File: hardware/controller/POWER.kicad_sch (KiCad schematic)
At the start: 22 parts, among them IC101 TPS63000IDRCRQ1, J101 1769

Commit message: done but need to add stitching vias
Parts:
- TP101, TP102, TP103, TP104, TP105: footprint TestPoint:TestPoint_Pad_1.0x1.0mm -> SamacSys_Parts:TestPoint_Pad_1.0x1.0mm
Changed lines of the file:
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@@
 			)
 		)
-		(property "Footprint" "TestPoint:TestPoint_Pad_1.0x1.0mm"
+		(property "Footprint" "SamacSys_Parts:TestPoint_Pad_1.0x1.0mm"
 			(at 190.5 62.23 0)
 			(effects
@@
 			)
 		)
-		(property "Footprint" "TestPoint:TestPoint_Pad_1.0x1.0mm"
+		(property "Footprint" "SamacSys_Parts:TestPoint_Pad_1.0x1.0mm"
 			(at 81.28 110.49 0)
 			(effects
@@
 			)
 		)
-		(property "Footprint" "TestPoint:TestPoint_Pad_1.0x1.0mm"
+		(property "Footprint" "SamacSys_Parts:TestPoint_Pad_1.0x1.0mm"
 			(at 81.28 71.12 0)
 			(effects
@@
 			)
 		)
-		(property "Footprint" "TestPoint:TestPoint_Pad_1.0x1.0mm"
+		(property "Footprint" "SamacSys_Parts:TestPoint_Pad_1.0x1.0mm"
 			(at 138.43 110.49 0)
 			(effects
@@
 			)
 		)
-		(property "Footprint" "TestPoint:TestPoint_Pad_1.0x1.0mm"
+		(property "Footprint" "SamacSys_Parts:TestPoint_Pad_1.0x1.0mm"
 			(at 190.5 72.39 0)
 			(effects

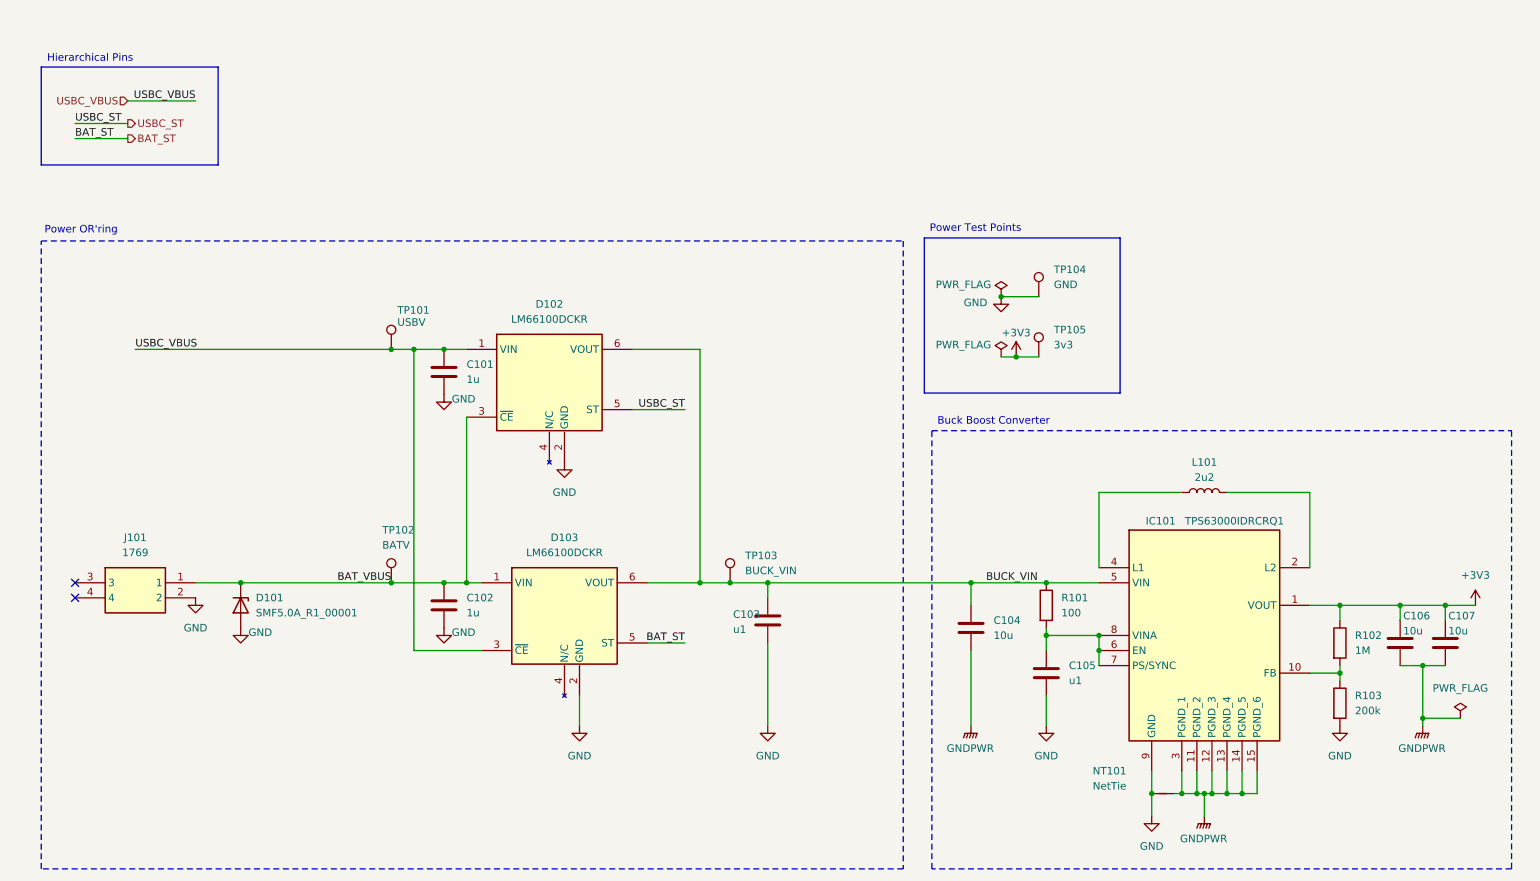
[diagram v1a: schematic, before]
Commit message: forgor
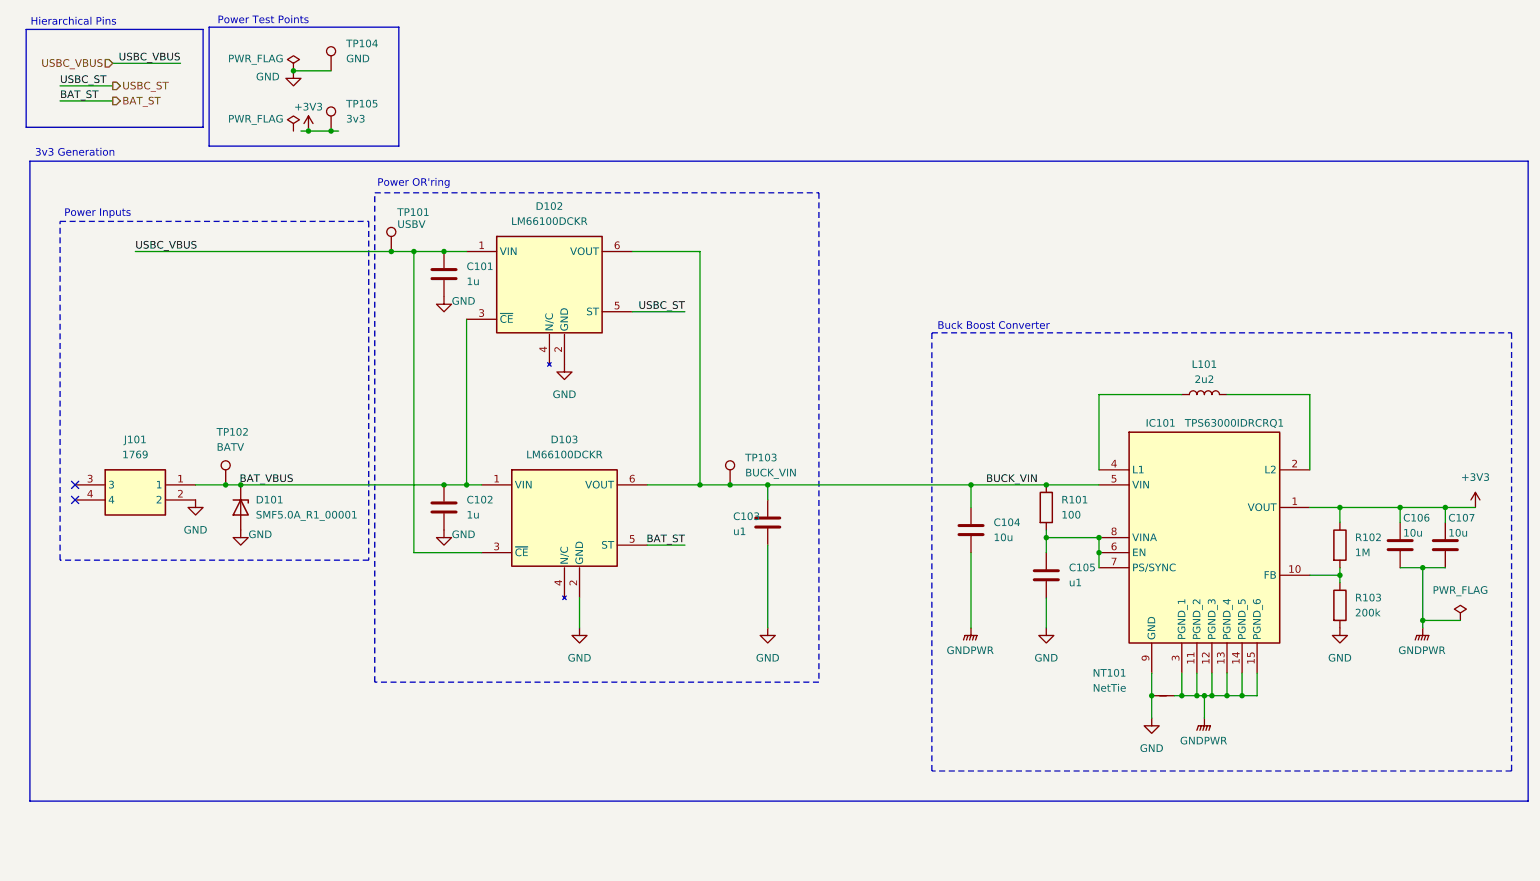
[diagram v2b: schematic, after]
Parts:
- NT101: footprint NetTie:NetTie-2_SMD_Pad0.5mm -> SamacSys_Parts:NetTie-2_Pad0.3mm
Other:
- note added: "3v3 Generation"
- note added: "Power Inputs"
- moved on the sheet: C101, C102, C103, C104, C105, C106, C107, D101, D102, D103, IC101, J101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
